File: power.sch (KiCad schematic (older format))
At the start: 14 parts, among them J1 Jack-DC, Q1 FDN340P, U1 NCP1117-5.0_SOT223, U2 LMV358IDGKR, U3 LP2985-3.3

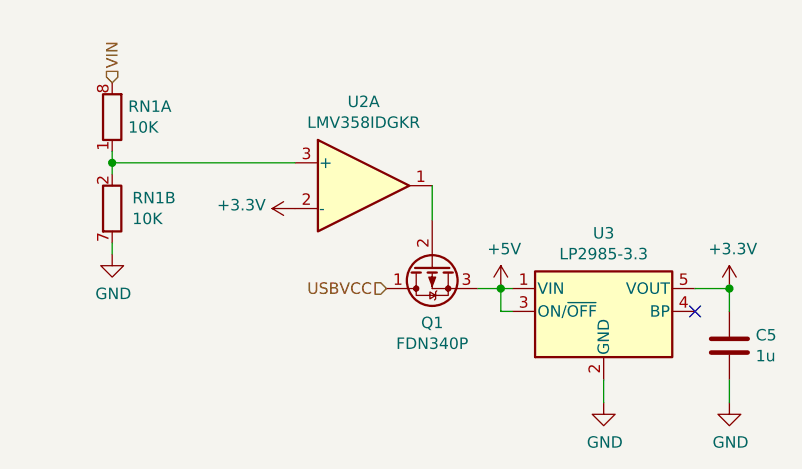
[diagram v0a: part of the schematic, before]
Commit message: update
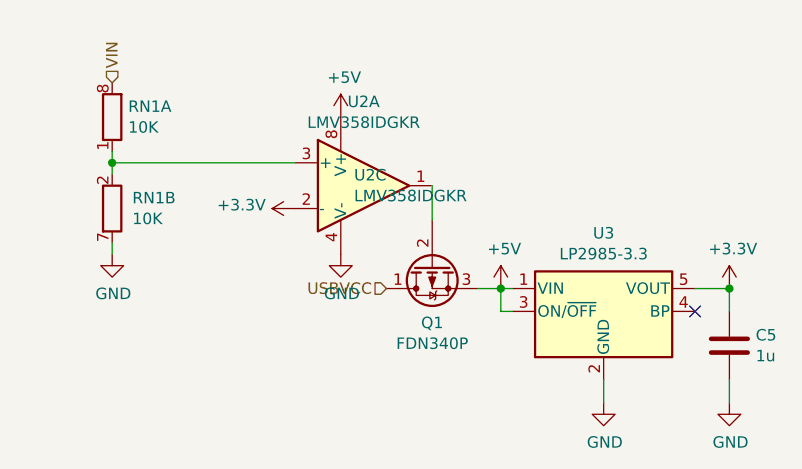
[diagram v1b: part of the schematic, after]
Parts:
- added unit 3 of U2
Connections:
- net +5V: now also U2.8 (V+)
- net GND: now also U2.4 (V-)
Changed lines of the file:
@@
 Wire Wire Line
 	3900 4750 3950 4750
+$Comp
+L Amplifier_Operational:LMV358 U2
+U 3 1 5C16AC1F
+P 7650 3300
+F 0 "U2" H 7608 3346 50  0000 L CNN
+F 1 "LMV358IDGKR" H 7608 3255 50  0000 L CNN
+F 2 "" H 7650 3300 50  0001 C CNN
+F 3 "http://www.ti.com/lit/ds/symlink/lmv324.pdf" H 7650 3300 50  0001 C CNN
+	3    7650 3300
+	1    0    0    -1
+$EndComp
+$Comp
+L power:+5V #PWR0102
+U 1 1 5C16B9F5
+P 7550 3000
+F 0 "#PWR0102" H 7550 2850 50  0001 C CNN
+F 1 "+5V" H 7565 3173 50  0000 C CNN
+F 2 "" H 7550 3000 50  0001 C CNN
+F 3 "" H 7550 3000 50  0001 C CNN
+	1    7550 3000
+	1    0    0    -1
+$EndComp
+$Comp
+L power:GND #PWR0103
+U 1 1 5C16BA9A
+P 7550 3600
+F 0 "#PWR0103" H 7550 3350 50  0001 C CNN
+F 1 "GND" H 7555 3427 50  0000 C CNN
+F 2 "" H 7550 3600 50  0001 C CNN
+F 3 "" H 7550 3600 50  0001 C CNN
+	1    7550 3600
+	1    0    0    -1
+$EndComp
 $EndSCHEMATC
